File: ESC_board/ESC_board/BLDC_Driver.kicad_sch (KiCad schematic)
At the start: 47 parts

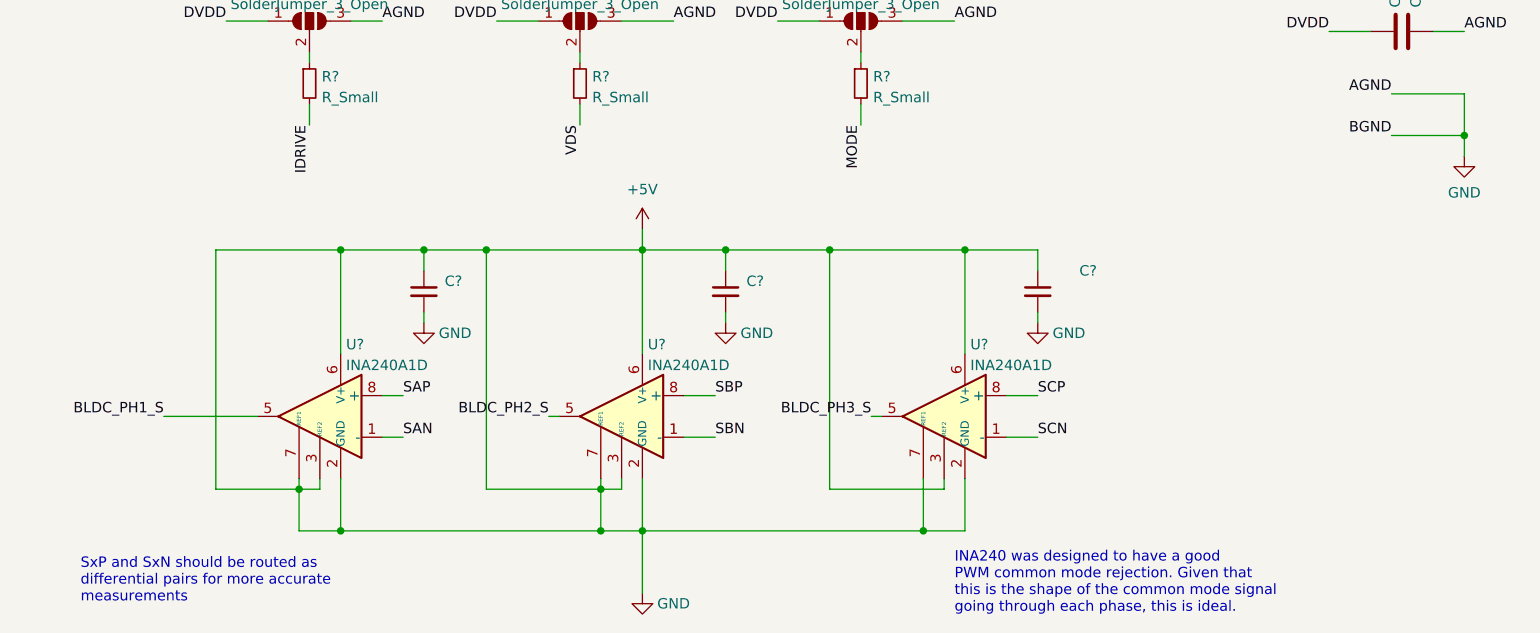
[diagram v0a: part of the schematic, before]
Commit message: Updated localization files
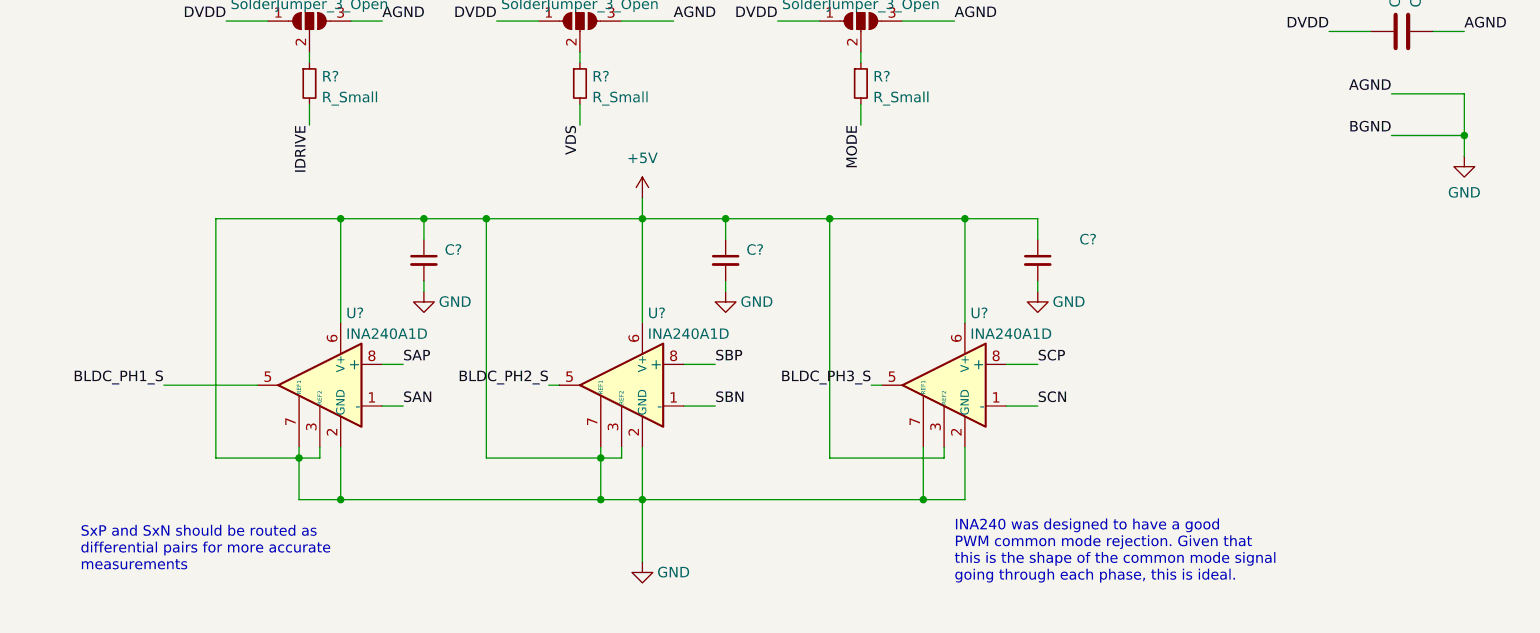
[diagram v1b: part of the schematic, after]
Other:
- moved on the sheet: C?, U?
